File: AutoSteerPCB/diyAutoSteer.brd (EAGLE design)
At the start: 127 x 99.1 mm, 65 parts, among them IC2 7805, IC3 7805, J1 I2C Out, J6 Reset, K4 CB1-P-12V, M1 ARDUINO-NANO-3.0, U2 ADC-4CH-ADS1115

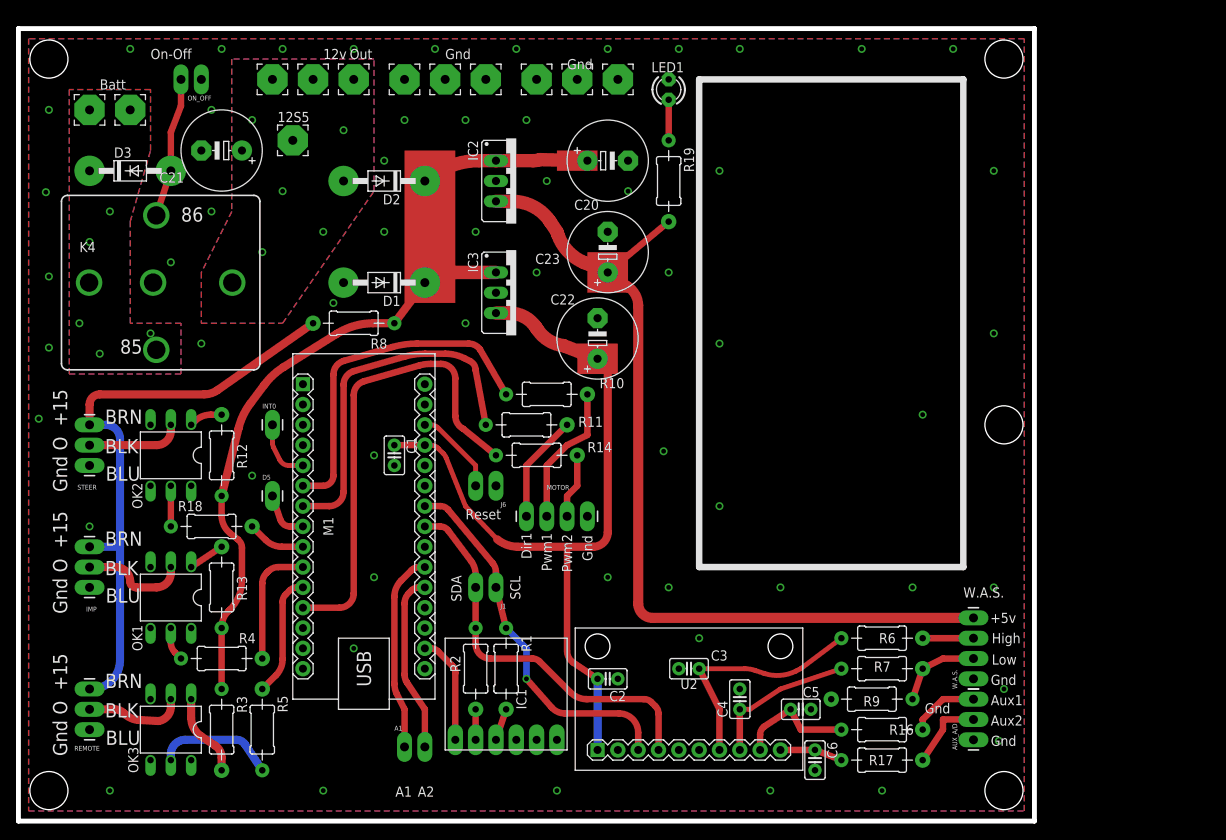
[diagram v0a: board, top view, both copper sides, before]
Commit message: v2 PCB
v2 PCB
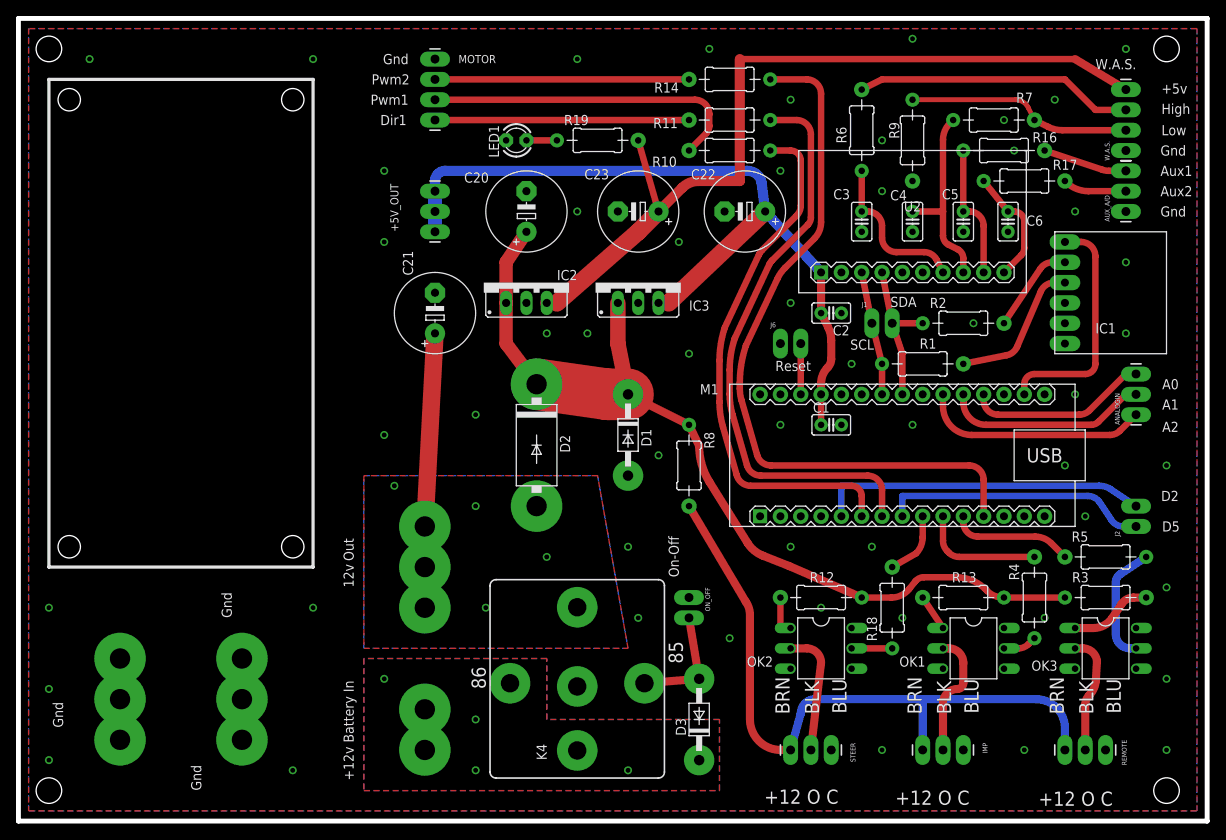
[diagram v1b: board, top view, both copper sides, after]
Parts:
- removed 12S5: WIREPAD3,81/1,1, wirepad:3,81/1,1
- removed A1: A2, SparkFun-Connectors:1X02_LONGPADS
- removed D5, INT0: (no value), SparkFun-Connectors:1X01_LONGPAD
- added +5V_OUT, ANALOGIN: (no value), SparkFun-Connectors:1X03_LONGPADS
- added J2: Pins, SparkFun-Connectors:1X02_LONGPADS
- D2: value 1N4004 -> 3A diode; device diode:DO41-10 -> diode:DO27-15
- moved REMOTE 127.0 mm to (135.9, 8.89), turned to 180 degrees
- moved OK3 117.3 mm to (135.9, 21.6), turned to 270 degrees
- moved R3 111.7 mm to (135.9, 27.9), turned to 0 degrees
- moved IMP 111.1 mm to (118.1, 8.89), turned to 180 degrees
- moved R5 107.6 mm to (135.9, 33.0), turned to 180 degrees
- moved R4 101.9 mm to (127.0, 27.9), turned to 90 degrees
- moved OK1 100.5 mm to (119.4, 21.6), turned to 270 degrees
- moved STEER 99.3 mm to (101.6, 8.89), turned to 180 degrees
- moved D3 98.8 mm to (85.1, 12.7), turned to 90 degrees
- moved GN5 95.5 mm to (12.7, 20.3), turned to 180 degrees
- moved GN4 94.4 mm to (12.7, 10.2)
- moved GN1 93.3 mm to (12.7, 15.2)
- moved R13 92.7 mm to (118.1, 27.9), turned to 180 degrees
- moved GN3 92.6 mm to (27.9, 10.2), turned to 0 degrees
- moved BAT1 90.3 mm to (50.8, 8.89), turned to 180 degrees
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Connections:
- removed net N$9: D5.1, M1.J1.8
- new net N$14: ANALOGIN.2, M1.J2.11
- new net N$18: J2.1, M1.J1.8
- net +5V: now also +5V_OUT.1, +5V_OUT.2, +5V_OUT.3
- net BATT: now also K4.86; no longer K4.85
- net N$10: now also ANALOGIN.3, M1.J2.12; no longer A1.1, M1.J2.10
- net N$15: now also ANALOGIN.1, M1.J2.10; no longer A1.2, M1.J2.11
- net N$24: now also K4.85; no longer K4.86
- net N$6: now also J2.2; no longer INT0.1
- net SW_RAW: no longer 12S5.1
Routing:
- net N$6: track 7.67 -> 41.3 mm
- net N$18: track 0.00 -> 33.3 mm
- net N$11: track 58.3 -> 89.5 mm
- net SCL: track 46.4 -> 15.5 mm, vias 1 -> 0
- net SDA: track 49.2 -> 19.4 mm
- net N$8: track 6.35 -> 34.9 mm
- net N$5: track 44.6 -> 71.9 mm
- net N$14: track 0.00 -> 25.2 mm
- net SW_RAW: track 0.00 -> 24.2 mm, vias 5 -> 4
- net N$21: track 8.15 -> 31.7 mm
- net N$4: track 43.1 -> 66.1 mm
- net N$17: track 17.9 -> 40.6 mm
- net N$19: track 13.5 -> 31.7 mm
- net N$2: track 10.7 -> 28.2 mm
- net N$1: track 13.6 -> 29.2 mm
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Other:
- board size 127 x 99.1 mm -> 148.6 x 100.3 mm
- board text added: "+12 O C"
- board text added: "+12v Battery In"
- board text added: "A0"
- board text added: "D2"
- board text added: "D5"
- board text removed: "+15"
- board text removed: "Batt"
- board text removed: "Gnd O"
